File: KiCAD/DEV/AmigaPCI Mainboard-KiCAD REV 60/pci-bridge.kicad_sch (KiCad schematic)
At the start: 43 parts, among them CN109 SPI, CN110 SPI, U109 ICE40HX4K-TQ144, U109F1 W25X20CLSN, U110 ICE40HX4K-TQ144, U110F1 W25X20CLSN

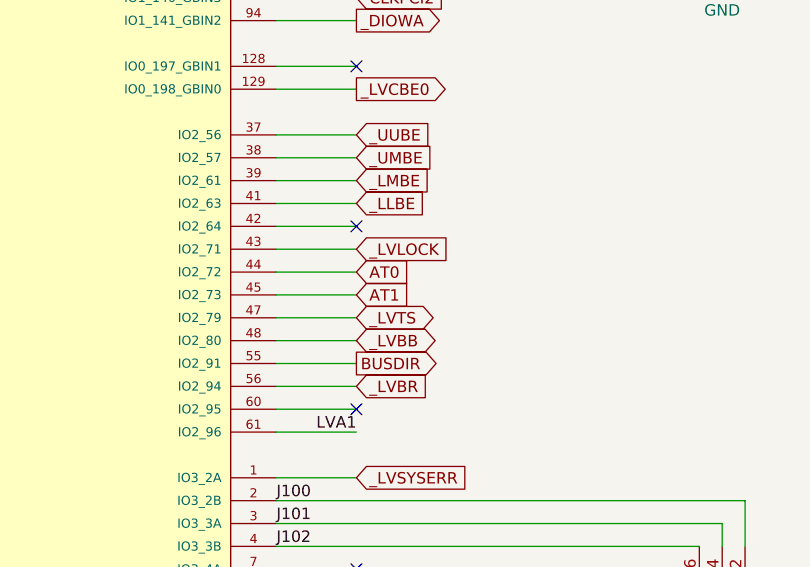
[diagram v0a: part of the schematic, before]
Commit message: APCI Rev 6.0 work.
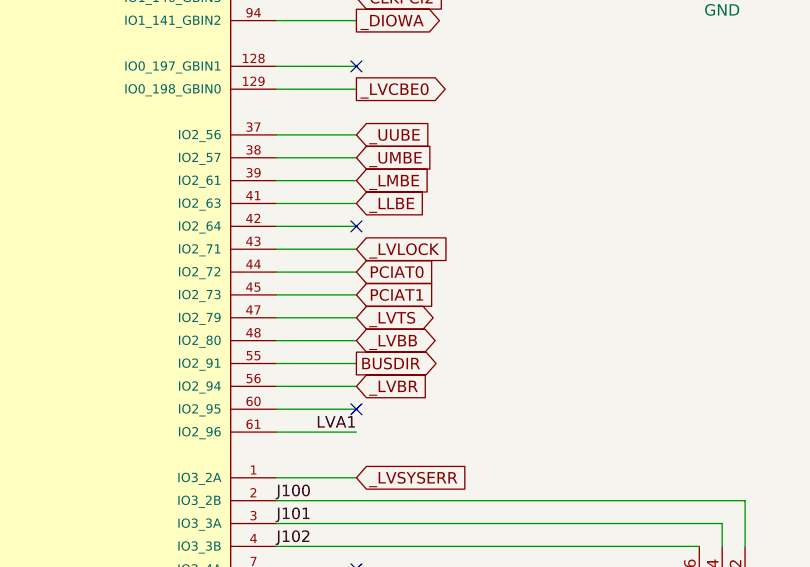
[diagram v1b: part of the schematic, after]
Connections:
- net AT0 renamed PCIAT0
- net AT1 renamed PCIAT1
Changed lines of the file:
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@@
 	(title_block
 		(title "AMIGA PCI")
-		(date "2025-05-24")
+		(date "2025-05-27")
 		(rev "6.0")
 	)
@@
 		)
 	)
-	(global_label "AT0"
+	(global_label "PCIAT0"
 		(shape input)
 		(at 281.94 129.54 0)
@@
 		)
 		(property "Intersheetrefs" "${INTERSHEET_REFS}"
-			(at 288.1909 129.54 0)
+			(at 291.3357 129.54 0)
 			(effects
 				(font
@@
 		)
 	)
-	(global_label "AT1"
+	(global_label "PCIAT1"
 		(shape input)
 		(at 281.94 132.08 0)
@@
 		)
 		(property "Intersheetrefs" "${INTERSHEET_REFS}"
-			(at 288.1909 132.08 0)
+			(at 291.3357 132.08 0)
 			(effects
 				(font
